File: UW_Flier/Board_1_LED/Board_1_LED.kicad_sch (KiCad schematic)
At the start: 13 parts, among them J1 RESET, J2 SWDIO, J3 SWDCLK, J4 GND, J5 VDD, J6 LED_DRAIN, Q1 CSD13385F5, U1 EYSHSNZWZ_module_stub, U2 BMP384

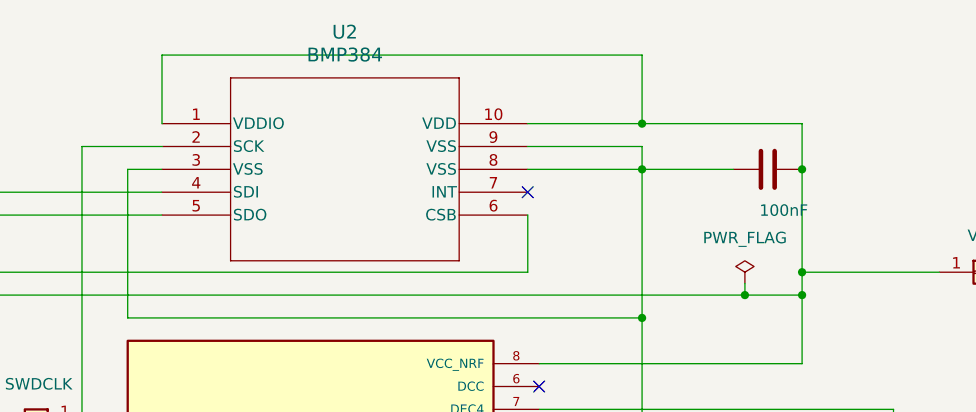
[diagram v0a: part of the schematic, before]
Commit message: stuff
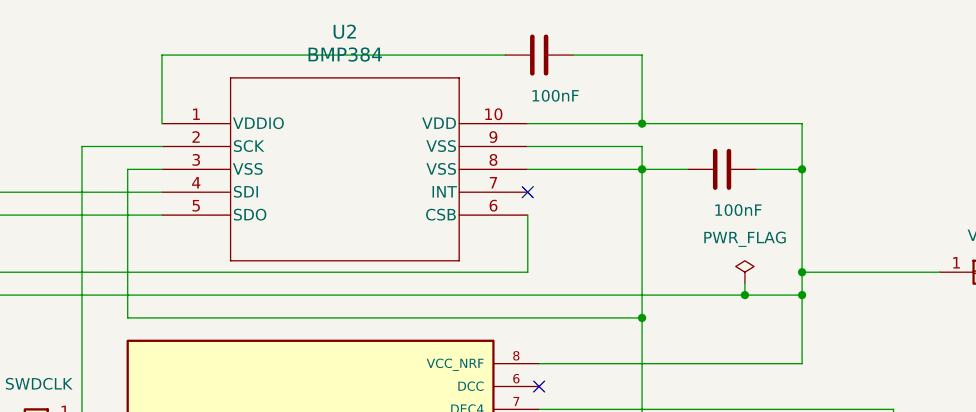
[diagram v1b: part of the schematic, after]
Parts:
- added C4: 100nF, Capacitor_SMD:C_0402_1005Metric, symbol Device:C
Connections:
- net at C1.1, C2.1, C6.2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: now also C4.2; no longer U2.1 (VDDIO)
- new net: C4.1, U2.1 (VDDIO)
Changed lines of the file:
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@@
 	(wire
 		(pts
-			(xy 118.11 30.48) (xy 107.95 30.48)
+			(xy 113.03 30.48) (xy 107.95 30.48)
 		)
 		(stroke
@@
 	(wire
 		(pts
+			(xy 120.65 30.48) (xy 125.73 30.48)
+		)
+		(stroke
+			(width 0)
+			(type default)
+		)
+	)
+	(wire
+		(pts
 			(xy 95.25 25.4) (xy 107.95 25.4)
 		)
@@
 	(wire
 		(pts
-			(xy 54.61 17.78) (xy 107.95 17.78)
+			(xy 54.61 17.78) (xy 92.71 17.78)
 		)
 		(stroke
@@
 		(pts
 			(xy 96.52 85.09) (xy 130.81 85.09)
+		)
+		(stroke
+			(width 0)
+			(type default)
+		)
+	)
+	(wire
+		(pts
+			(xy 100.33 17.78) (xy 107.95 17.78)
 		)
 		(stroke
@@
 	(symbol
 		(lib_id "Device:C")
-		(at 121.92 30.48 90)
+		(at 116.84 30.48 90)
 		(unit 1)
 		(exclude_from_sim no)
@@
 		(dnp no)
 		(property "Reference" "C6"
-			(at 118.92 30.48 0)
+			(at 113.84 30.48 0)
 			(effects
 				(font
@@
 		)
 		(property "Value" "100nF"
-			(at 123.698 35.052 90)
+			(at 118.618 35.052 90)
 			(effects
 				(font
@@
 		)
 		(property "Footprint" "Capacitor_SMD:C_0402_1005Metric"
-			(at 125.73 29.5148 0)
+			(at 120.65 29.5148 0)
 			(effects
 				(font
@@
 		)
 		(property "Datasheet" "~"
-			(at 121.92 30.48 0)
+			(at 116.84 30.48 0)
 			(effects
 				(font
@@
 		)
 		(property "Description" "Unpolarized capacitor"
-			(at 121.92 30.48 0)
+			(at 116.84 30.48 0)
 			(effects
 				(font
@@
 					(unit 1)
 				)
+			)
+		)
+	)
+	(symbol
+		(lib_id "Device:C")
+		(at 96.52 17.78 90)
+		(unit 1)
+		(exclude_from_sim no)
+		(in_bom yes)
+		(on_board yes)
+		(dnp no)
+		(property "Reference" "C4"
+			(at 93.52 17.78 0)
+			(effects
+				(font
+					(size 1.27 1.27)
+				)
+				(hide yes)
+			)
+		)
+		(property "Value" "100nF"
+			(at 98.298 22.352 90)
+			(effects
+				(font
+					(size 1.27 1.27)
+				)
+			)
+		)
+		(property "Footprint" "Capacitor_SMD:C_0402_1005Metric"
+			(at 100.33 16.8148 0)
+			(effects
+				(font
+					(size 1.27 1.27)
+				)
+				(hide yes)
+			)
+		)
+		(property "Datasheet" "~"
+			(at 96.52 17.78 0)
+			(effects
+				(font
+					(size 1.27 1.27)
+				)
+				(hide yes)
+			)
+		)
+		(property "Description" "Unpolarized capacitor"
+			(at 96.52 17.78 0)
+			(effects
+				(font
+					(size 1.27 1.27)
+				)
+				(hide yes)
+			)
+		)
+		(pin "2"
+		)
+		(pin "1"
+		)
+		(instances
+			(project "Board_1_LED"
+				(path "/3845d15c-5f8e-47c3-ba57-143dd1318a5f"
+					(reference "C4")
+					(unit 1)
+				)
